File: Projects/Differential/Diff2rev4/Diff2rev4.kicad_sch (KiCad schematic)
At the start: 43 parts, among them J1 AVR-ISP-6, J3 12401598E4_2A, U1 ATmega32U4-M, U2 DRV8904QPWPRQ1, U3 AP7363-33D-13, Y1 C5S-24.000-20-3030-X-R

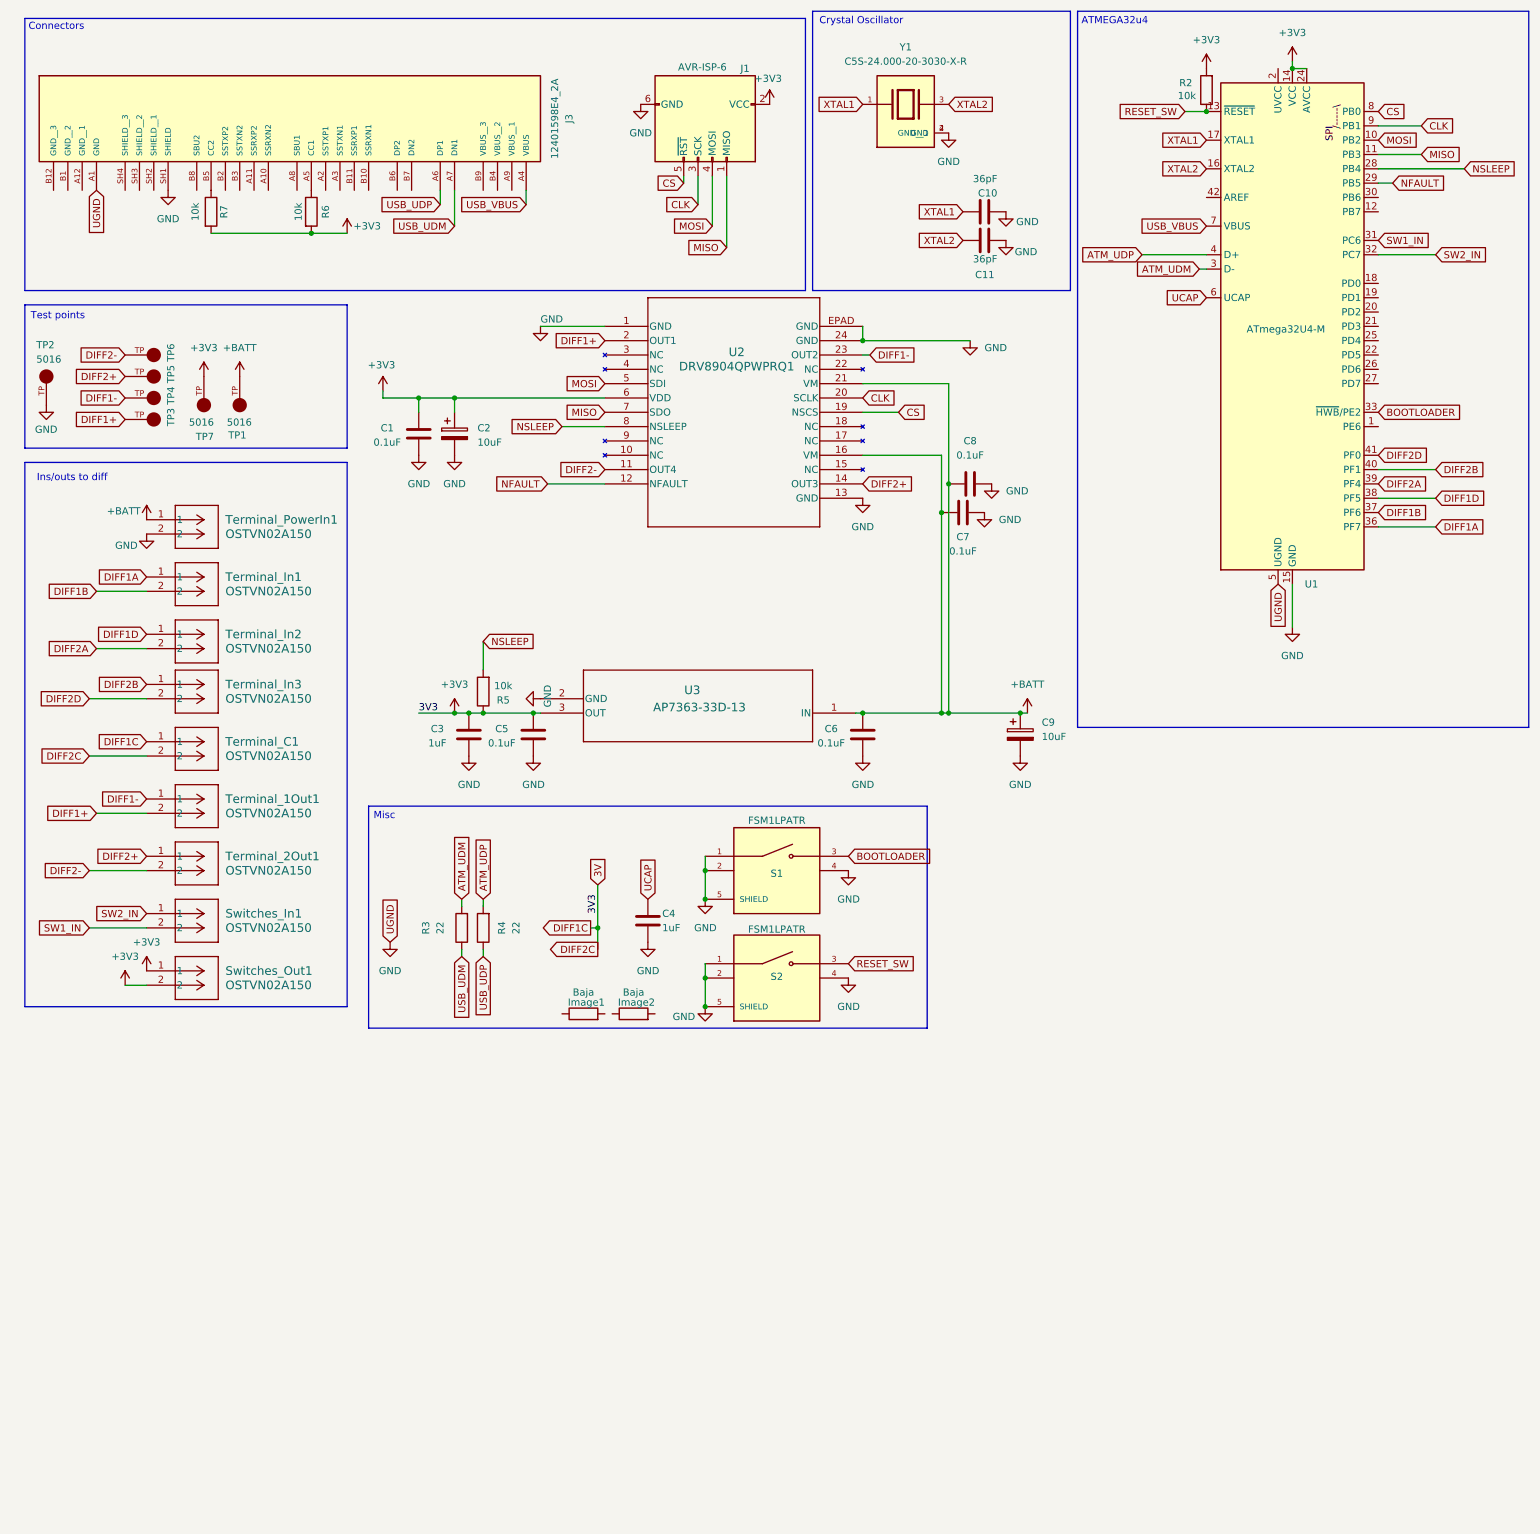
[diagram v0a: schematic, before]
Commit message: chore: clean kicad schematics
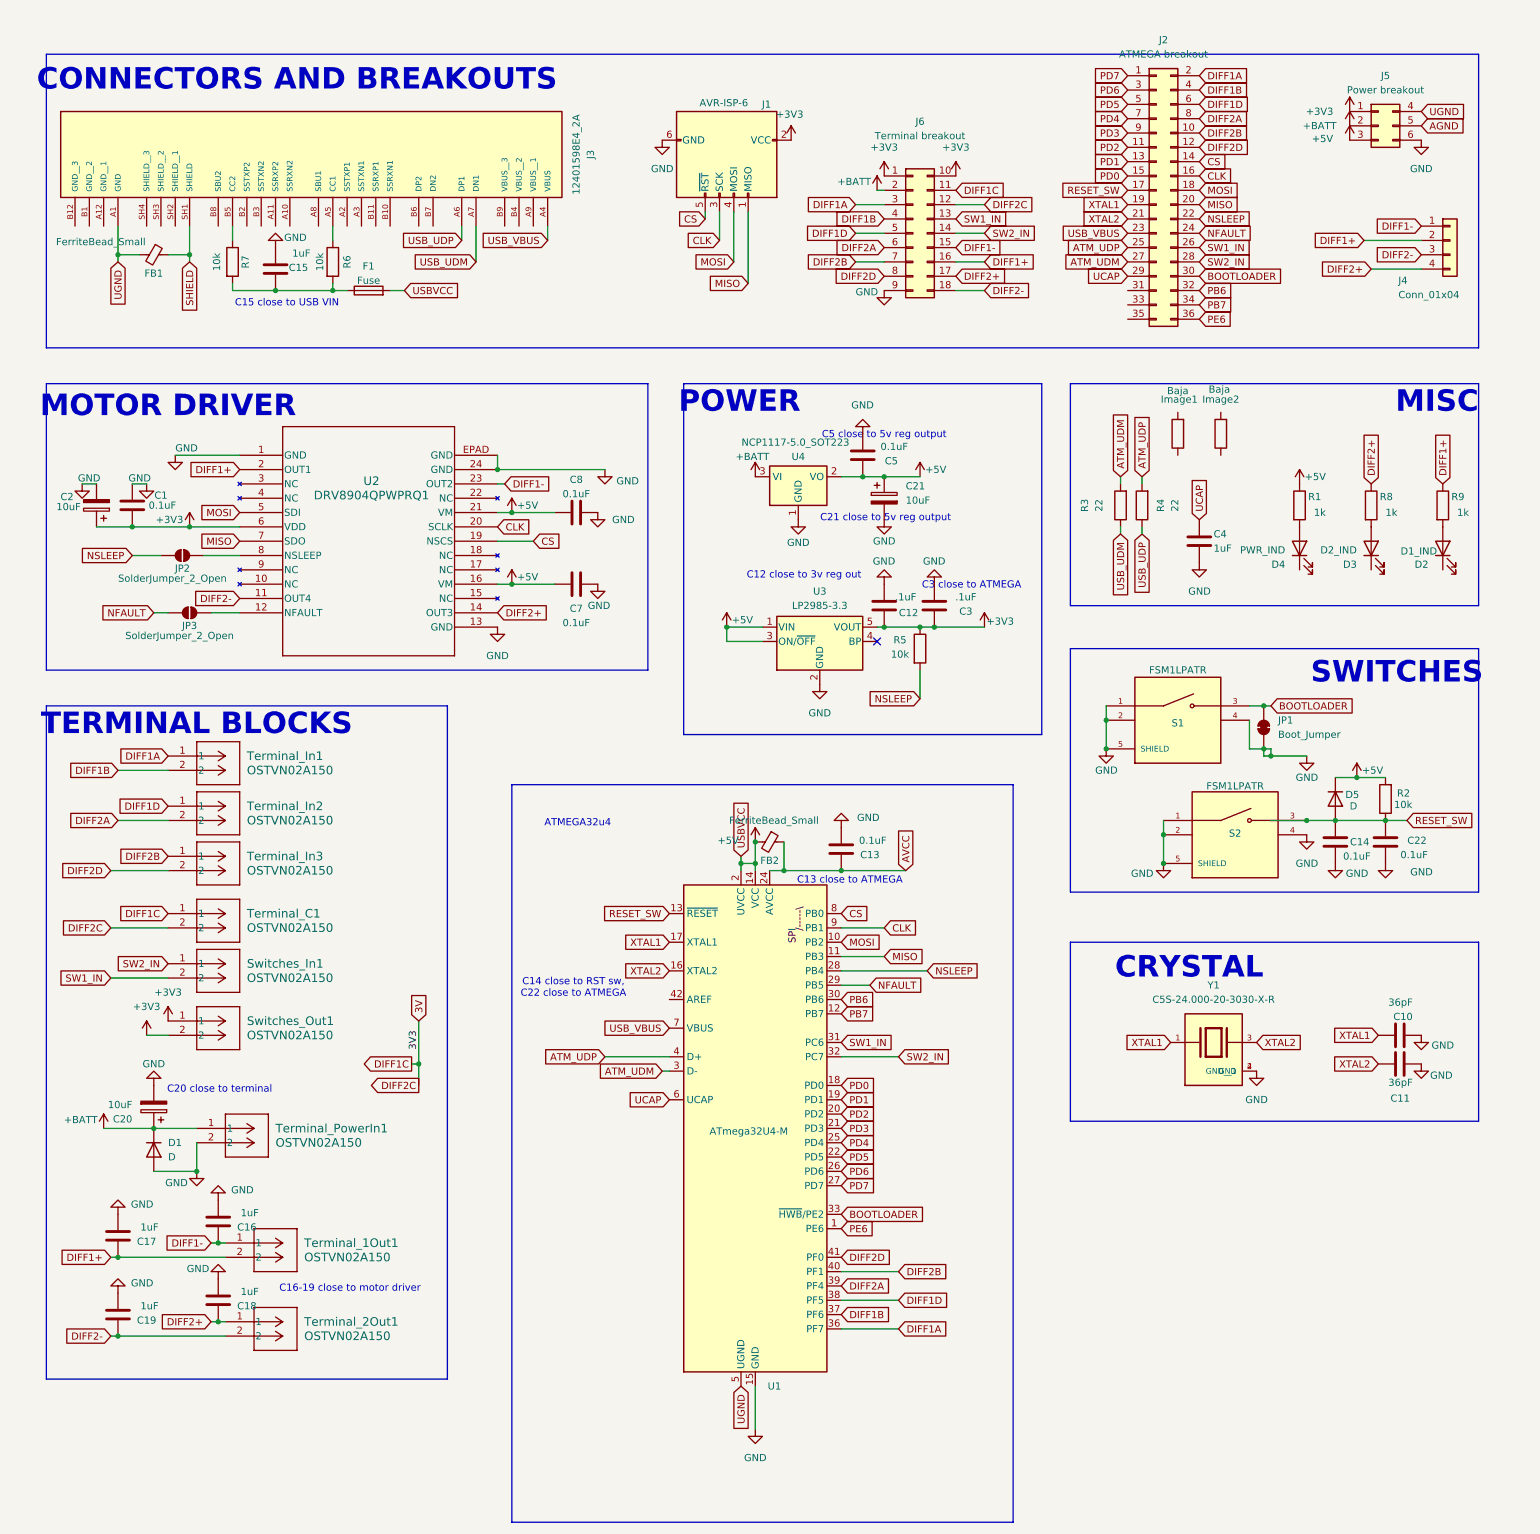
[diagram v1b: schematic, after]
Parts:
- removed C6: 0.1uF, Capacitor_SMD:C_0805_2012Metric, symbol Device:C
- removed C9: 10uF, Capacitor_SMD:C_0805_2012Metric, symbol Device:C_Polarized
- removed TP1, TP2, TP3, TP4, TP5, TP6, TP7: 5016, custom:KEYSTONE_5016, symbol custom:5016
- removed U3: AP7363-33D-13, Package_TO_SOT_SMD:TO-252-2, symbol 2025-05-12_01-07-32:AP7363-33D-13
- added C12: .1uF, Capacitor_SMD:C_0805_2012Metric, symbol Device:C
- added C13, C14, C22: 0.1uF, Capacitor_SMD:C_0805_2012Metric, symbol Device:C
- added C15, C16, C17, C18, C19: 1uF, Capacitor_SMD:C_0805_2012Metric, symbol Device:C
- added C20, C21: 10uF, Capacitor_SMD:C_0805_2012Metric, symbol Device:C_Polarized
- added D1, D5: D, symbol Device:D
- added D2: D1_IND, symbol Device:LED
- added D3: D2_IND, symbol Device:LED
- added D4: PWR_IND, symbol Device:LED
- added F1: Fuse, symbol Device:Fuse
- added FB1, FB2: FerriteBead_Small, symbol Device:FerriteBead_Small
- added J2: ATMEGA breakout, symbol Connector_Generic:Conn_02x18_Odd_Even
- added J4: Conn_01x04, symbol Connector_Generic:Conn_01x04
- added J5: Power breakout, symbol Connector_Generic:Conn_02x03_Top_Bottom
- added J6: Terminal breakout, symbol Connector_Generic:Conn_02x09_Top_Bottom
- added JP1: Boot_Jumper, symbol Jumper:SolderJumper_2_Bridged
- added JP2, JP3: SolderJumper_2_Open, symbol Jumper:SolderJumper_2_Open
- added R1, R8, R9: 1k, symbol Device:R
- added U3: LP2985-3.3, Package_TO_SOT_SMD:SOT-23-5, symbol Regulator_Linear:LP2985-3.3
- added U4: NCP1117-5.0_SOT223, Package_TO_SOT_SMD:SOT-223-3_TabPin2, symbol Regulator_Linear:NCP1117-5.0_SOT223
- C3: value 1uF -> .1uF
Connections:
- net +3V3: now also C12.1, J5.1 (Pin_1), J6.1 (Pin_1), J6.10 (Pin_10), U3.5 (VOUT); no longer C5.1, R2.2, R6.2, R7.2, Terminal_C1.1, Terminal_C1.2, U1.14 (VCC), U1.24 (AVCC), U1.34 (VCC), U1.44 (AVCC)
- net +BATT: now also C20.1, D1.1 (K), J5.2 (Pin_2), J6.2 (Pin_2), U4.3 (VI); no longer C7.1, C8.1, U2.16 (VM), U2.21 (VM)
- net ATM_UDM: now also J2.27 (Pin_27)
- net ATM_UDP: now also J2.25 (Pin_25)
- net BOOTLOADER: now also J2.30 (Pin_30), JP1.2 (B)
- net CLK: now also J2.16 (Pin_16)
- net CS: now also J2.14 (Pin_14)
- net DIFF1+: now also C17.1, J4.2 (Pin_2), J6.16 (Pin_16), R9.1
- net DIFF1-: now also C16.1, J4.1 (Pin_1), J6.15 (Pin_15)
- net DIFF1A: now also J2.2 (Pin_2), J6.3 (Pin_3)
- net DIFF1B: now also J2.4 (Pin_4), J6.4 (Pin_4)
- net DIFF1D: now also J2.6 (Pin_6), J6.5 (Pin_5)
- net DIFF2+: now also C18.1, J4.4 (Pin_4), J6.17 (Pin_17), R8.1
- net DIFF2-: now also C19.1, J4.3 (Pin_3), J6.18 (Pin_18)
- net DIFF2A: now also J2.8 (Pin_8), J6.6 (Pin_6)
- net DIFF2B: now also J2.10 (Pin_10), J6.7 (Pin_7)
- net DIFF2D: now also J2.12 (Pin_12), J6.8 (Pin_8)
- net GND: now also C12.2, C13.2, C14.2, C15.2, C16.2, C17.2, C18.2, C19.2, C20.2, C21.2, C22.2, D1.2 (A), J5.6 (Pin_6), J6.9 (Pin_9), JP1.1 (A), U3.2 (GND), U4.1 (GND); no longer J3.A1 (GND), J3.SH1 (SHIELD), U1.5 (UGND)
- net MISO: now also J2.20 (Pin_20)
- net MOSI: now also J2.18 (Pin_18)
- net NFAULT: now also J2.24 (Pin_24), JP3.1 (A); no longer U2.12 (NFAULT)
- net NSLEEP: now also J2.22 (Pin_22), JP2.1 (A); no longer U2.8 (NSLEEP)
- net RESET_SW: now also C14.1, C22.1, D5.2 (A), J2.17 (Pin_17)
- net SW1_IN: now also J2.26 (Pin_26), J6.13 (Pin_13)
- net SW2_IN: now also J2.28 (Pin_28), J6.14 (Pin_14)
- net UCAP: now also J2.29 (Pin_29)
- net USB_VBUS: now also J2.23 (Pin_23)
- net XTAL1: now also J2.19 (Pin_19)
- net XTAL2: now also J2.21 (Pin_21)
- net PE6: now reaches U1.1 (PE6)
- net PE6: now also J2.36 (Pin_36)
- net PB7: now reaches U1.12 (PB7)
- net PB7: now also J2.34 (Pin_34)
- net PD0: now reaches U1.18 (PD0)
- net PD0: now also J2.15 (Pin_15)
- net PD1: now reaches U1.19 (PD1)
- net PD1: now also J2.13 (Pin_13)
- net +5V: now reaches U1.2 (UVCC)
- net +5V: now also C5.1, C7.1, C8.1, R2.2, U1.14 (VCC), U1.34 (VCC), U2.16 (VM), U2.21 (VM), C21.1, D5.1 (K), F1.2, FB2.2, J5.3 (Pin_3), R1.1, U3.1 (VIN), U3.3 (ON/~{OFF}), U4.2 (VO)
- net PD2: now reaches U1.20 (PD2)
- net PD2: now also J2.11 (Pin_11)
- net PD3: now reaches U1.21 (PD3)
- net PD3: now also J2.9 (Pin_9)
- net PD5: now reaches U1.22 (PD5)
- net PD5: now also J2.5 (Pin_5)
- net PD4: now reaches U1.25 (PD4)
- net PD4: now also J2.7 (Pin_7)
- net PD6: now reaches U1.26 (PD6)
- net PD6: now also J2.3 (Pin_3)
- net PD7: now reaches U1.27 (PD7)
- net PD7: now also J2.1 (Pin_1)
- net PB6: now reaches U1.30 (PB6)
- net PB6: now also J2.32 (Pin_32)
- new net: JP3.2 (B), U2.12 (NFAULT)
- new net: D3.2 (A), R8.2
- new net: D2.2 (A), R9.2
- new net: C15.1, F1.1, R6.2, R7.2
- new net: JP2.2 (B), U2.8 (NSLEEP)
- new net: D4.2 (A), R1.2
- new net 3V: J6.11 (Pin_11), J6.12 (Pin_12), Terminal_C1.1, Terminal_C1.2
- new net AGND: J5.5 (Pin_5)
- new net AVCC: C13.1, FB2.1, U1.24 (AVCC), U1.44 (AVCC)
- new net SHIELD: FB1.1, J3.SH1 (SHIELD)
- new net UGND: FB1.2, J3.A1 (GND), J5.4 (Pin_4), U1.5 (UGND)
- no-connect marks 0 -> 1
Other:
- note added: "C12 close to 3v reg out"
- note added: "C13 close to ATMEGA"
- note added: "C14 close to RST sw, C22 close to ATMEGA"
- note added: "C15 close to USB VIN"
- note added: "C16-19 close to motor driver"
- note added: "C20 close to terminal"
- note added: "C21 close to 5v reg output"
- note added: "C3 close to ATMEGA"
- note added: "C5 close to 5v reg output"
- note added: "CONNECTORS AND BREAKOUTS"
- note added: "CRYSTAL"
- note added: "MISC"
- note added: "MOTOR DRIVER"
- note added: "POWER"
- note added: "SWITCHES"
- note added: "TERMINAL BLOCKS"
- note removed: "Connectors"
- note removed: "Crystal Oscillator"
- note removed: "Ins/outs to diff"
- note removed: "Misc"
- note removed: "Test points"
- moved on the sheet: C1, C10, C11, C2, C3, C4, C5, C7, C8, Image1, Image2, J1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
